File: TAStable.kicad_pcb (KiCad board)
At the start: 2 copper layers, 20 x 16.5 mm, 12 parts, among them J1 Conn_01x06_Pin, U1 74AHCT1G04, U2 CS2300-CP, U3 74LVC1G14

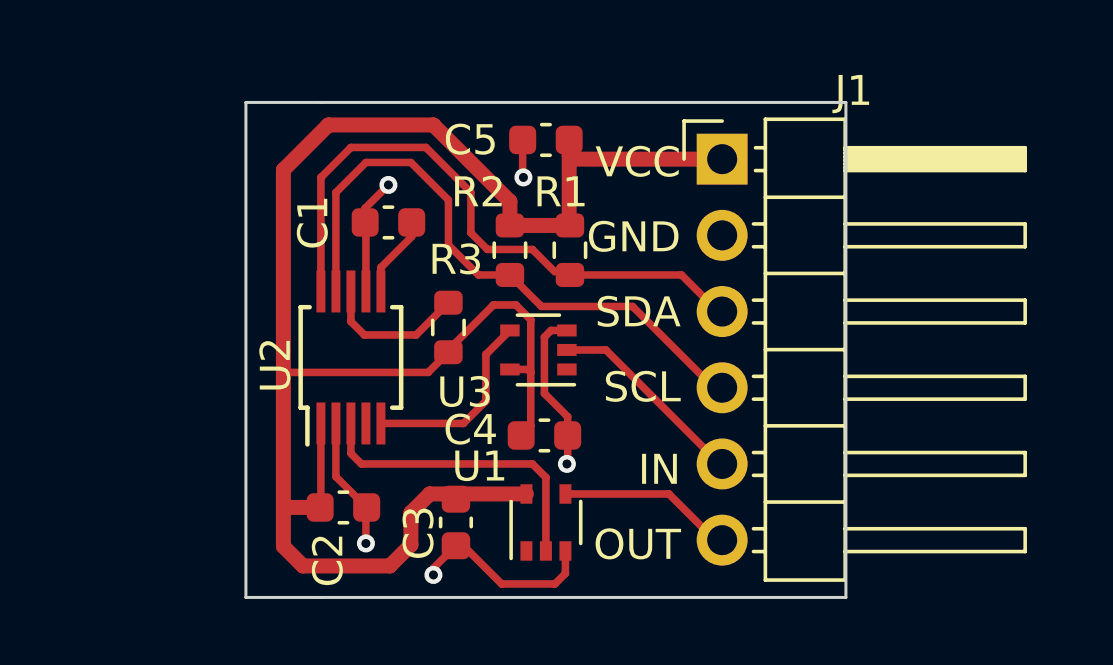
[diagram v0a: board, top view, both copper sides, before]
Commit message: cleanups
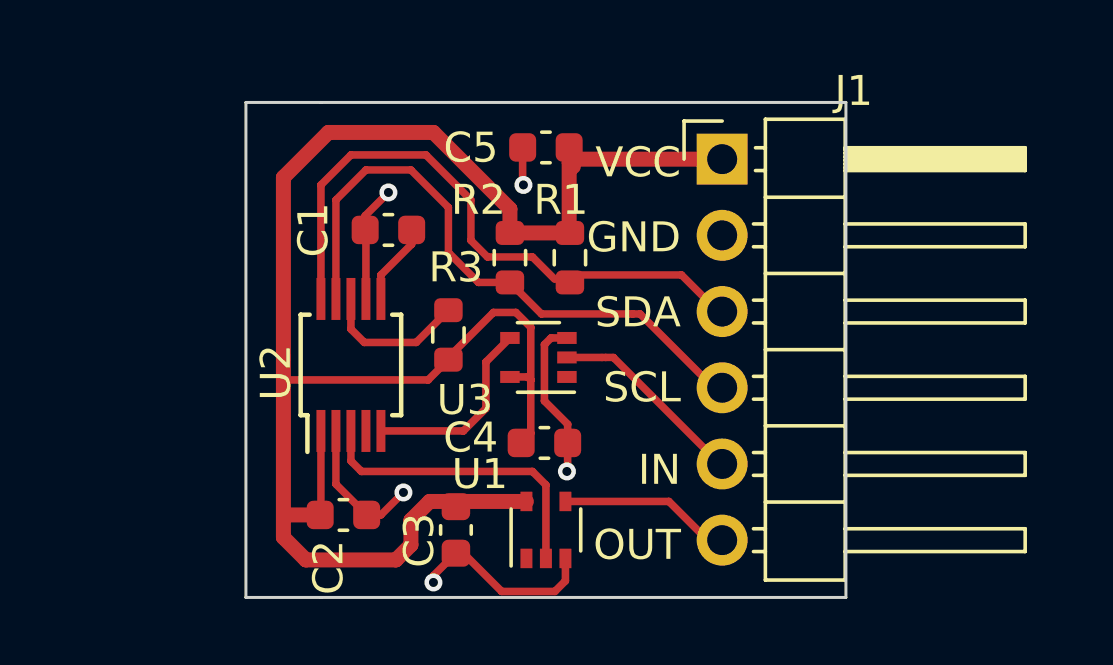
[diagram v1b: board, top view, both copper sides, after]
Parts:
- moved C1 0.25 mm to (129.2, 96.0)
- moved C2 0.25 mm to (127.8, 105.5)
- moved C3 0.25 mm to (131.5, 106.0)
- moved C4 0.25 mm to (134.4, 103.1)
- moved C5 0.25 mm to (134.5, 93.2)
- moved R1 0.25 mm to (135.3, 96.9)
- moved R2 0.25 mm to (133.3, 96.9)
- moved R3 0.25 mm to (131.2, 99.5)
- moved U1 0.25 mm to (134.5, 106.0)
- moved U2 0.25 mm to (128.0, 100.5)
- moved U3 0.25 mm to (134.2, 100.2)
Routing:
- net +3.3V: track 61.0 -> 60.2 mm
- added copper zone on F.Cu, net GND

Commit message: code!
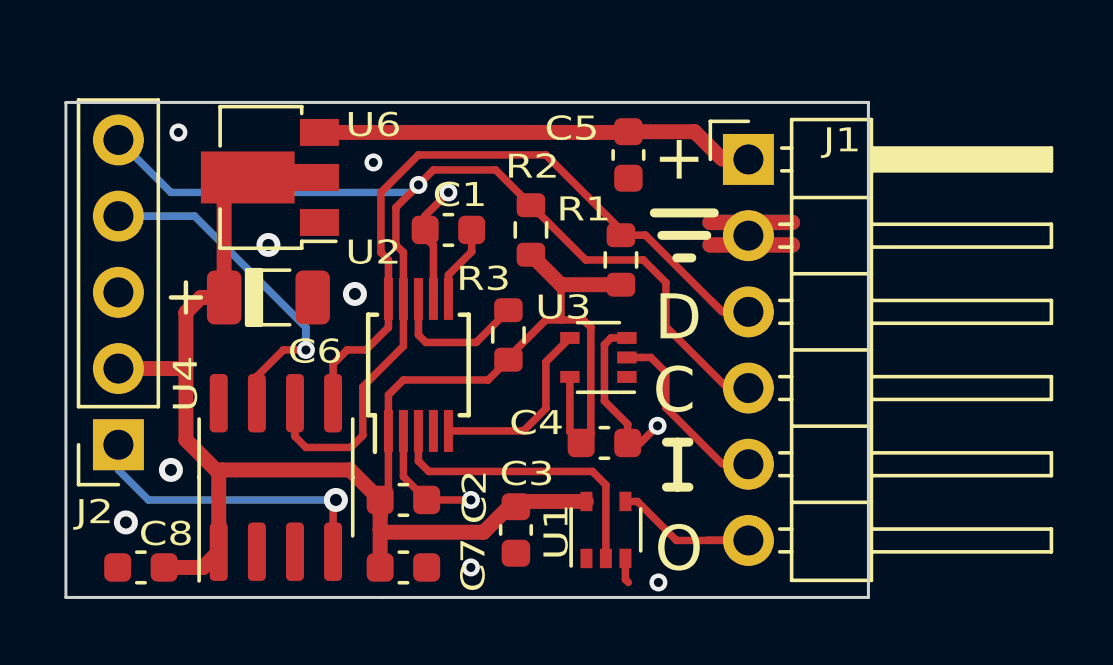
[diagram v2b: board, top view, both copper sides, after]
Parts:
- added C6: 22uF Tantalum, Capacitor_SMD:C_1206_3216Metric, F.Cu at (125.2, 98.2)
- added C7: 1uF, Capacitor_SMD:C_0603_1608Metric, F.Cu at (129.8, 107.2)
- added C8: 100nF, Capacitor_SMD:C_0603_1608Metric, F.Cu at (121.0, 107.2)
- added J2: ICSP, Connector_PinSocket_2.54mm:PinSocket_1x05_P2.54mm_Vertical, F.Cu at (120.2, 103.2)
- added U4: PIC16LF15313, Package_SO:SOIC-8_3.9x4.9mm_P1.27mm, F.Cu at (125.5, 104.2)
- added U6: AZ1117-3.3, Package_TO_SOT_SMD:SOT-89-3, F.Cu at (125.0, 94.2)
- U1: value 74AHCT1G04 -> 74HCT1G04
- moved C5 2.76 mm to (137.2, 93.5), turned to -90 degrees
- moved U2 2.25 mm to (130.2, 100.5)
- moved C2 2.06 mm to (129.8, 105.0)
- moved C1 2.00 mm to (131.2, 96.0)
- moved C3 2.00 mm to (133.5, 106.0)
- moved C4 2.00 mm to (136.4, 103.1)
- moved R3 2.00 mm to (133.2, 99.5)
- moved U1 2.00 mm to (136.5, 106.0)
- moved U3 2.00 mm to (136.2, 100.2)
- moved R1 1.70 mm to (137.0, 97.0), turned to 90 degrees
- moved R2 1.16 mm to (134.0, 96.0), turned to 90 degrees
- moved J1 0.88 mm to (141.2, 93.7)
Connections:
- C5 pad 1: +3.3V -> +5V
- J1 pad 1: +3.3V -> +5V
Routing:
- net /I2C_SCL: track 20.6 -> 38.9 mm, vias 0 -> 1
- net +5V: track 0.00 -> 13.8 mm
- net /ICSPDAT: track 0.00 -> 11.4 mm, vias 0 -> 1
- net /MCLR: track 0.00 -> 10.3 mm, vias 0 -> 1
- net GND: track 21.8 -> 25.4 mm, vias 5 -> 11
- net /I2C_SDA: track 20.2 -> 23.1 mm
- net Net-(J1-Pin_6): track 5.76 -> 4.25 mm
- net /21MHz_IN: track 6.65 -> 5.33 mm
- net +3.3V: track 60.2 -> 59.3 mm
- net Net-(U2-CLK_IN): track 7.04 -> 6.24 mm
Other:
- board size 20 x 16.5 mm -> 26.8 x 16.5 mm
- board text added: "+"
- board text added: "C"
- board text added: "D"
- board text added: "O"
- board text added: "github/ rasteri/ TAStable"
